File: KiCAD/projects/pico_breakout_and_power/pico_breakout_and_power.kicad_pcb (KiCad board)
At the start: 2 copper layers, 46 x 59.7 mm, 14 parts, among them IC1 STCS05DR, J1 Conn_01x05_Socket

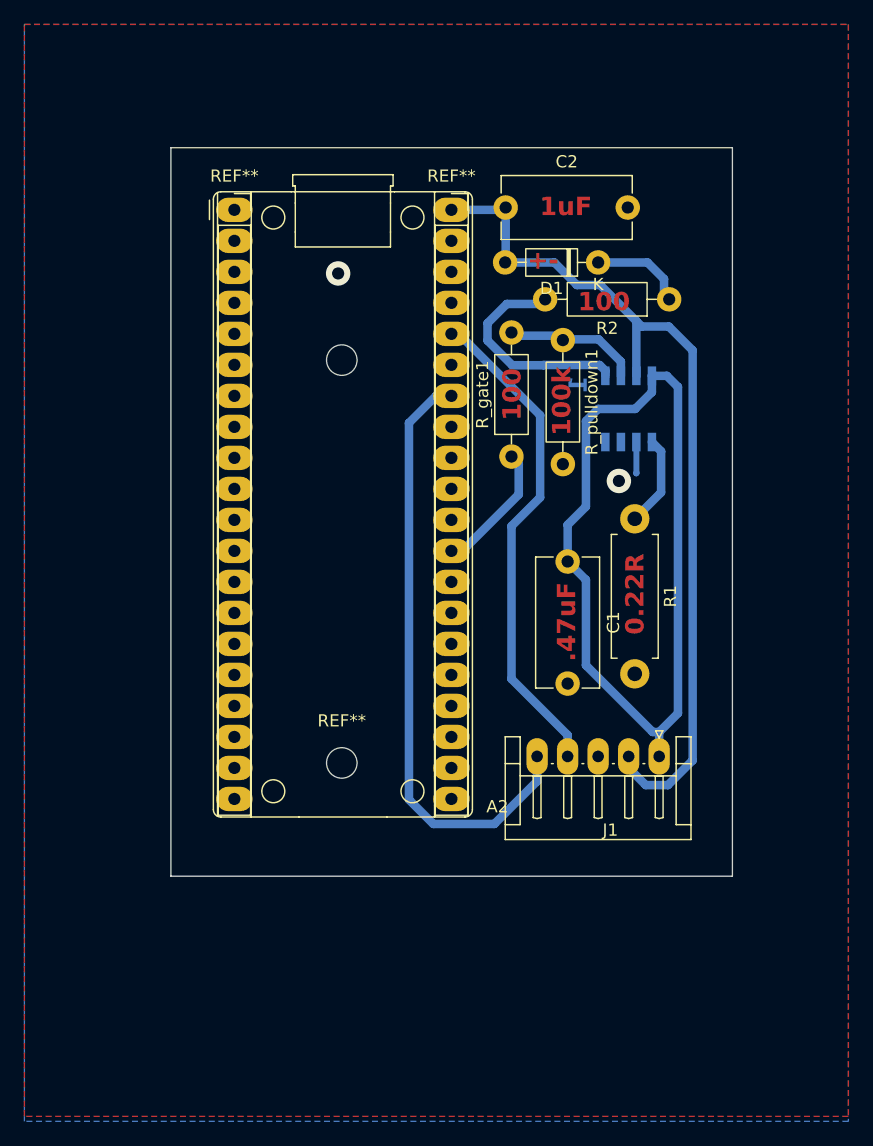
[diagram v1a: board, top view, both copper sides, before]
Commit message: Final Pico breakout board.
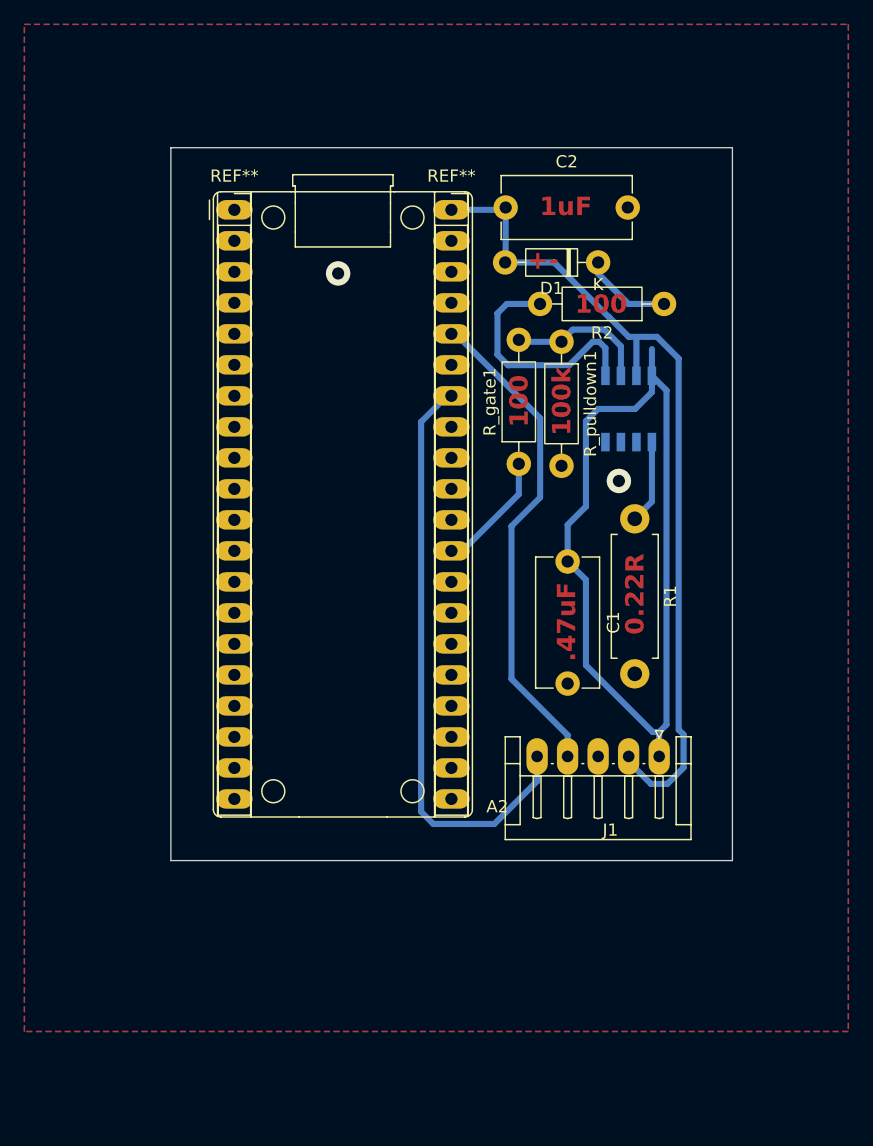
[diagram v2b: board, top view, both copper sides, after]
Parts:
- removed ?: , 
- removed the REF** at (136.0, 103.0)
- moved R_gate1 0.85 mm to (150.5, 78.5)
- moved R2 0.57 mm to (162.4, 65.4)
- moved R_pulldown1 0.18 mm to (154.0, 68.5)
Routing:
- net /VBUS_5V/ANODE: track 73.3 -> 69.8 mm
- net GND: track 2.57 -> 0.00 mm
- net Net-(IC1-VCC): track 18.1 -> 19.7 mm
- net /GPIO28_ADC2: track 50.1 -> 48.7 mm
- net /GPIO22: track 10.8 -> 9.94 mm
- net /Cathode: track 70.7 -> 71.4 mm
- net Net-(IC1-PWM): track 11.2 -> 11.9 mm
- net Net-(IC1-FB): track 7.50 -> 6.87 mm
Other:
- board size 46 x 59.7 mm -> 46 x 58.4 mm
- board text removed: "1"
